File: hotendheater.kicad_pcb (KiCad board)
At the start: 2 copper layers, 43.8 x 63.2 mm, 13 parts, among them J1 Conn_01x02_Pin, J2 Conn_01x02_Pin, J3 Conn_01x08_Socket, J4 Conn_01x02_Pin, J5 Conn_01x02_Pin, Q1 IRF540N

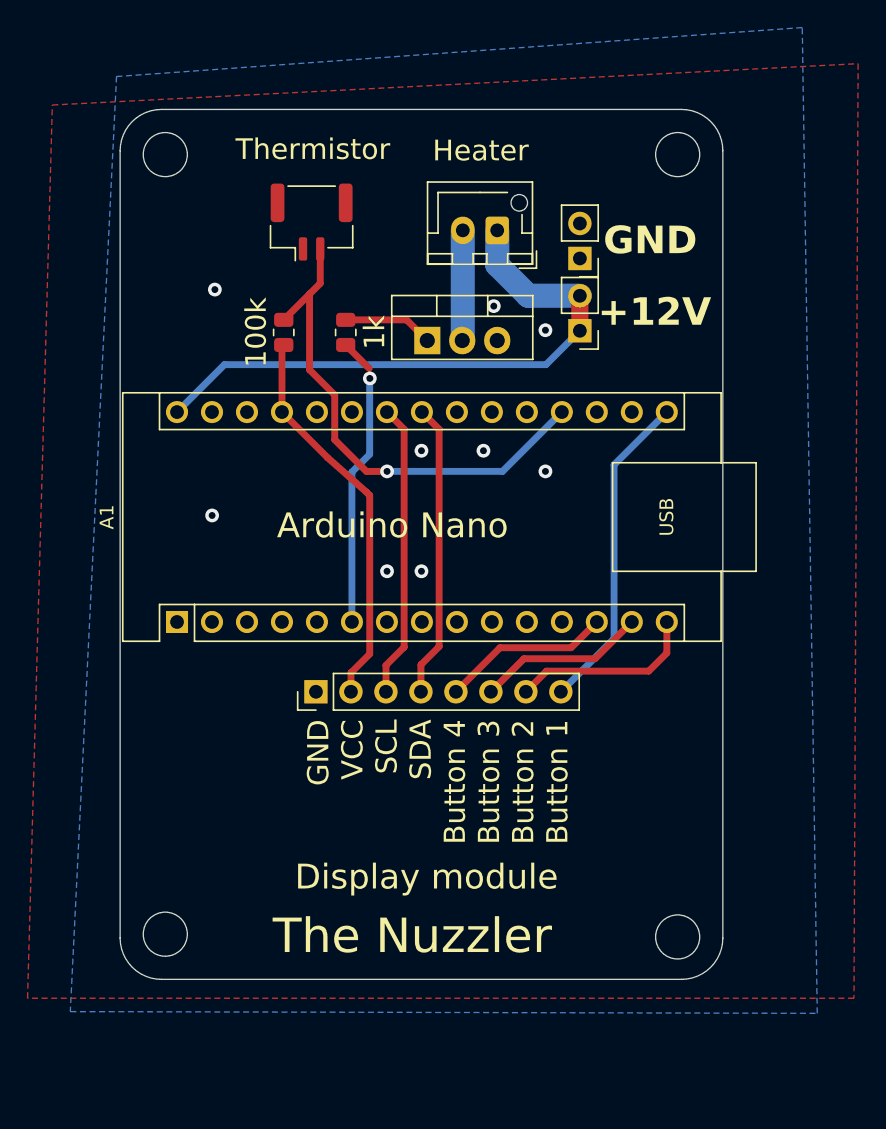
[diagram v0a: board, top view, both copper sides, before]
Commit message: Improvements
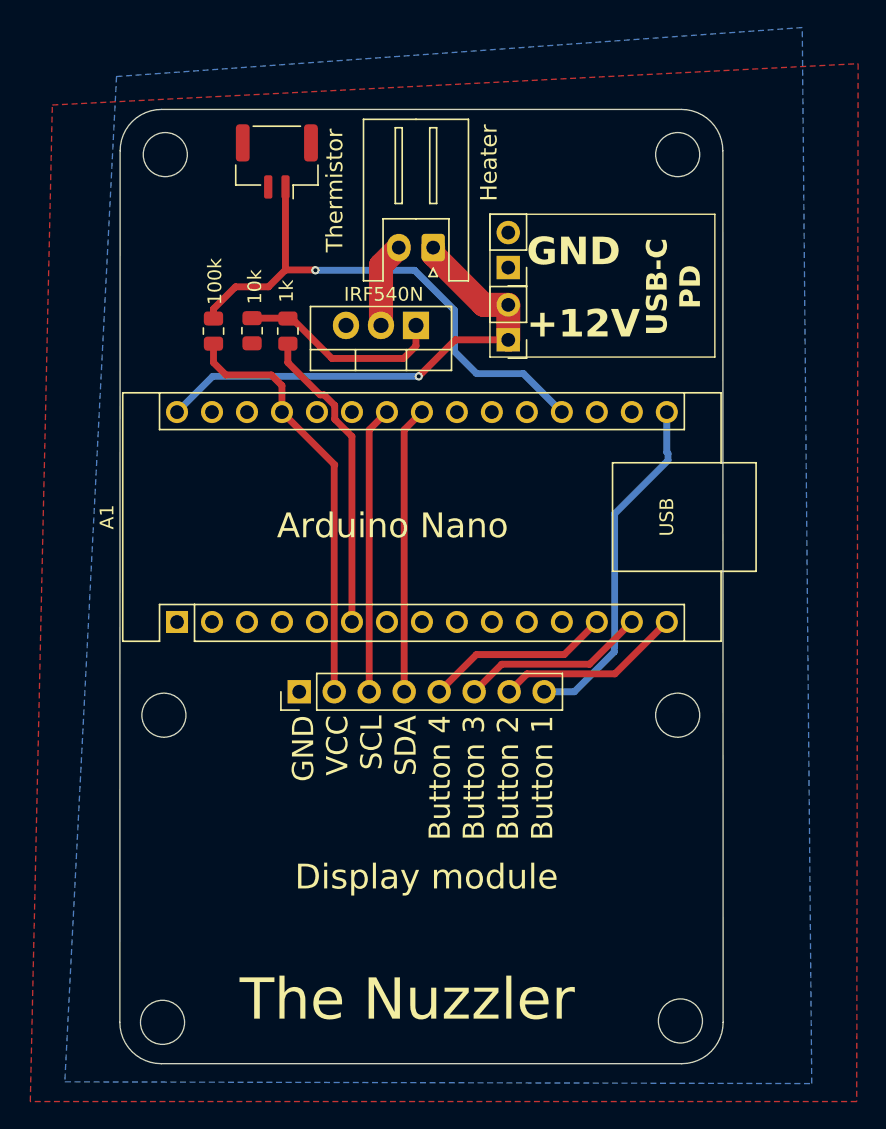
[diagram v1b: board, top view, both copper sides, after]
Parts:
- removed J2: Conn_01x02_Pin, Connector_JST:JST_GH_BM02B-GHS-TBT_1x02-1MP_P1.25mm_Vertical
- added H5: MountingHole, MountingHole:MountingHole_3.2mm_M3_DIN965, F.Cu at (110.3, 105.7)
- added H6: MountingHole, MountingHole:MountingHole_3.2mm_M3_DIN965, F.Cu at (147.6, 105.7)
- added J6: Conn_01x02_Shielded, Connector_JST:JST_GH_SM02B-GHS-TB_1x02-1MP_P1.25mm_Horizontal, F.Cu at (118.5, 65.5)
- added R3: 10k, Resistor_SMD:R_0805_2012Metric, F.Cu at (116.7, 77.8)
- J1: footprint Connector_JST:JST_XH_B2B-XH-AM_1x02_P2.50mm_Vertical -> Connector_JST:JST_XH_S2B-XH-A_1x02_P2.50mm_Horizontal
- moved H2 6.40 mm to (110.2, 128.0)
- moved H4 6.10 mm to (147.8, 127.9)
- moved J4 5.24 mm to (135.3, 78.5)
- moved J5 5.24 mm to (135.3, 73.2)
- moved R2 5.10 mm to (113.9, 77.8)
- moved J1 4.82 mm to (129.8, 71.8)
- moved R1 4.20 mm to (119.3, 77.8)
- moved Q1 1.37 mm to (128.6, 77.4), turned to 180 degrees
- moved J3 1.22 mm to (120.1, 104.0)
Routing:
- net Net-(Q1-G): track 6.54 -> 15.0 mm
- net +12V: track 43.7 -> 36.2 mm, vias 0 -> 1
- net /Thermistor: track 36.8 -> 39.2 mm
- net +5V: track 28.5 -> 30.9 mm
- net /Button1: track 23.5 -> 25.4 mm
- net Net-(J1-Pin_2): track 8.02 -> 6.18 mm
- net /Heater: track 20.6 -> 22.3 mm, vias 1 -> 0
- net /Button3: track 12.3 -> 13.5 mm
- net /Button4: track 12.3 -> 13.5 mm
- net /SDA: track 21.4 -> 20.8 mm
- net /SCL: track 21.4 -> 20.8 mm
- net GND: vias 9 -> 0
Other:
- board size 43.8 x 63.2 mm -> 43.8 x 69.3 mm
- board text added: "USB-C PD"
